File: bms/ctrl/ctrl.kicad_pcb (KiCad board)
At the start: 2 copper layers, 1 part

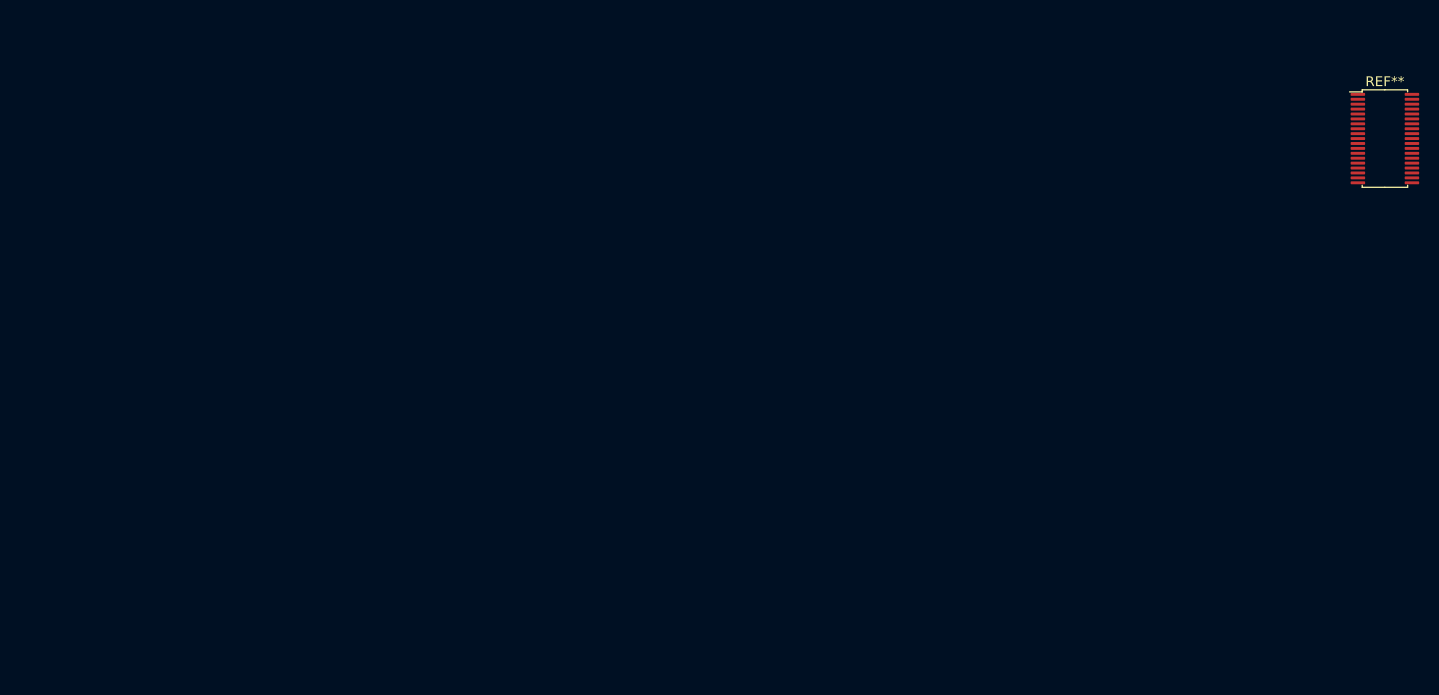
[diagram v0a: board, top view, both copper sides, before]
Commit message: BMS stuff update
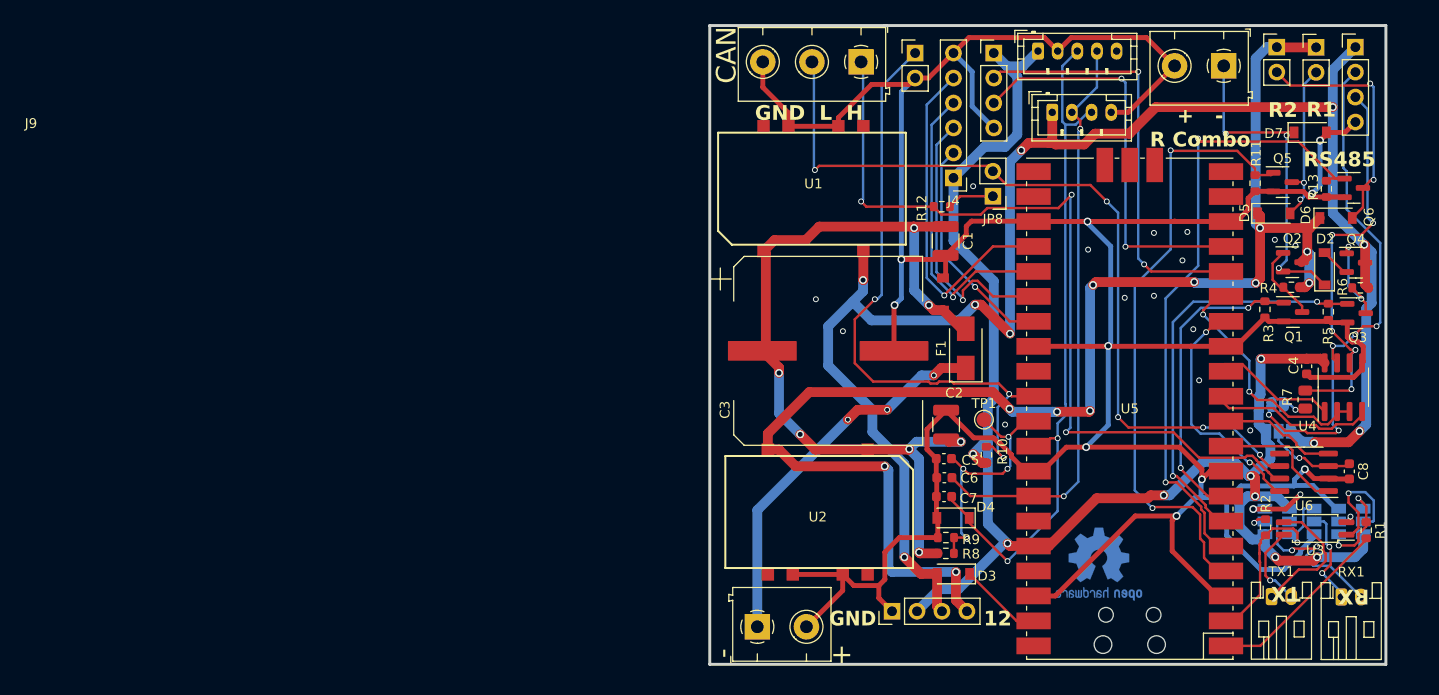
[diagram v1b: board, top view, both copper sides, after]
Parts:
- removed the REF** at (111.9, 82.9)
- added C1: CP_1µ_100V_0805, Resistor_SMD:R_1210_3225Metric, F.Cu at (67.2, 93.3)
- added C2: CP_1µ_100V_0805, Resistor_SMD:R_1210_3225Metric, F.Cu at (67.2, 112.0)
- added C3: CP_330µ_100V_1210, localstuff:CP_Elec_19x19, F.Cu at (55.2, 104.5)
- added C4: 100nF, Capacitor_SMD:C_0603_1608Metric, F.Cu at (103.9, 106.1)
- added C5: CP_100n_50V_0603, Capacitor_SMD:C_0603_1608Metric, F.Cu at (67.0, 115.5)
- added C6: CP_100n_50V_0603, Capacitor_SMD:C_0603_1608Metric, F.Cu at (67.1, 117.4)
- added C7: CP_100n_50V_0603, Capacitor_SMD:C_0603_1608Metric, F.Cu at (67.0, 119.3)
- added C8: CP_10µ_16V_0603, Capacitor_SMD:C_0603_1608Metric, F.Cu at (108.3, 116.8)
- added D1: D_TVS_70V, localstuff:SOD-123FL, F.Cu at (66.9, 98.7)
- added D2: 1N4148, Diode_SMD:D_SOD-123, F.Cu at (105.8, 96.2)
- added D3: D_Schottky, Diode_SMD:D_SOD-123, F.Cu at (68.0, 127.2)
- added D4: D_Zener_3V3, Diode_SMD:D_SOD-123, F.Cu at (68.0, 121.5)
- added D5: 1N4148, Diode_SMD:D_SOD-123, F.Cu at (100.6, 90.5)
- added D6: 1N4148, Diode_SMD:D_SOD-123, F.Cu at (106.9, 91.0)
- added D7: 1N4148, Diode_SMD:D_SOD-123, F.Cu at (104.3, 82.3)
- added F1: Polyfuse 100V, Diode_SMD:D_SMA, F.Cu at (69.2, 104.2)
- added J1: Conn_01x02_Female, localstuff:Conn_P5.0mm_2_Lumberg, F.Cu at (48.0, 132.6)
- added J10: Conn_LEM_3, Connector_JST:JST_PH_B5B-PH-K_1x05_P2.00mm_Vertical, F.Cu at (76.6, 74.0)
- added J11: Conn_01x02_Female, Connector_PinHeader_2.54mm:PinHeader_1x02_P2.54mm_Vertical, F.Cu at (100.9, 73.6)
- added J12: Conn_01x04, Connector_PinHeader_2.54mm:PinHeader_1x04_P2.54mm_Vertical, F.Cu at (61.8, 131.0)
- added J2: Conn_01x02_Female, localstuff:Conn_P5.0mm_2_Lumberg, F.Cu at (95.5, 75.5)
- added J3: ScrewTerminal, Connector_PinHeader_2.54mm:PinHeader_1x04_P2.54mm_Vertical, F.Cu at (108.9, 73.6)
- added J4: Conn_01x06, Connector_PinHeader_2.54mm:PinHeader_1x06_P2.54mm_Vertical, F.Cu at (68.0, 86.9)
- added J5: Conn_01x04, Connector_PinHeader_2.54mm:PinHeader_1x04_P2.54mm_Vertical, F.Cu at (72.1, 74.2)
- added J6: Conn_LEM_5, Connector_JST:JST_PH_B4B-PH-K_1x04_P2.00mm_Vertical, F.Cu at (78.0, 80.2)
- added J7: Conn_01x02_Male, Connector_PinHeader_2.54mm:PinHeader_1x02_P2.54mm_Vertical, F.Cu at (64.1, 74.2)
- added J8: Conn_01x02_Female, Connector_PinHeader_2.54mm:PinHeader_1x02_P2.54mm_Vertical, F.Cu at (104.9, 73.6)
- added J9: Conn_01x03, localstuff:Conn_P5.0mm_3_Lumberg, F.Cu at (58.6, 75.1)
- added JP1: SolderJumper_3_Bridged12, Jumper:SolderJumper-3_P1.3mm_Open_Pad1.0x1.5mm, B.Cu at (109.7, 121.9)
- added JP2: SolderJumper_3_Bridged12, Jumper:SolderJumper-3_P1.3mm_Open_Pad1.0x1.5mm, B.Cu at (107.2, 121.9)
- added JP3: SolderJumper_3_Bridged12, Jumper:SolderJumper-3_P1.3mm_Open_Pad1.0x1.5mm, B.Cu at (102.2, 121.9)
- added JP4: SolderJumper_3_Bridged12, Jumper:SolderJumper-3_P1.3mm_Open_Pad1.0x1.5mm, B.Cu at (104.7, 121.9)
- added JP5: SolderJumper_3_Bridged12, Jumper:SolderJumper-3_P1.3mm_Open_Pad1.0x1.5mm, B.Cu at (99.7, 121.9)
- added JP6: OptTermination, Jumper:SolderJumper-2_P1.3mm_Open_RoundedPad1.0x1.5mm, B.Cu at (101.0, 110.0)
- added JP7: CANBUS Volt Select, Jumper:SolderJumper-3_P1.3mm_Bridged12_RoundedPad1.0x1.5mm, B.Cu at (101.1, 112.7)
- added JP8: Jumper_2_Open, Connector_PinHeader_2.54mm:PinHeader_1x02_P2.54mm_Vertical, F.Cu at (72.0, 88.8)
- added Q1: DMN2058U-7, Package_TO_SOT_SMD:SOT-23, F.Cu at (102.5, 100.5)
- added Q2: XP221P0501TR-G, Package_TO_SOT_SMD:SOT-23, F.Cu at (102.5, 95.5)
- added Q3: DMN2058U-7, Package_TO_SOT_SMD:SOT-23, F.Cu at (109.0, 100.7)
- added Q4: XP221P0501TR-G, Package_TO_SOT_SMD:SOT-23, F.Cu at (109.0, 95.5)
- added Q5: DMN2058U-7, Package_TO_SOT_SMD:SOT-23, F.Cu at (101.5, 87.3)
- added Q6: DMN2058U-7, Package_TO_SOT_SMD:SOT-23, F.Cu at (108.7, 87.9)
- added R1: R_220_0603, Resistor_SMD:R_0603_1608Metric, F.Cu at (110.0, 122.8)
- added R10: R_10k_0603, Resistor_SMD:R_0603_1608Metric, F.Cu at (71.3, 115.1)
- added R11: R_1M_0603, Resistor_SMD:R_0603_1608Metric, F.Cu at (98.7, 87.4)
- added R12: R_120_0603, Resistor_SMD:R_0603_1608Metric, F.Cu at (66.8, 89.8)
- added R13: R_1M_0603, Resistor_SMD:R_0603_1608Metric, F.Cu at (106.0, 88.0)
- added R2: R_2k2_0603, Resistor_SMD:R_0603_1608Metric, F.Cu at (99.8, 122.5)
- added R3: R_1M_0603, Resistor_SMD:R_0603_1608Metric, F.Cu at (99.7, 100.3)
- added R4: R_1M_0603, Resistor_SMD:R_0603_1608Metric, F.Cu at (102.4, 98.0)
- added R5: R_1M_0603, Resistor_SMD:R_0603_1608Metric, F.Cu at (106.1, 100.5)
- added R6: R_1M_0603, Resistor_SMD:R_0603_1608Metric, F.Cu at (109.4, 98.1)
- added R7: 120R, Resistor_SMD:R_0805_2012Metric, F.Cu at (103.8, 109.5)
- added R8: R_750k_0603, Resistor_SMD:R_0603_1608Metric, F.Cu at (67.2, 125.1)
- added R9: R_36k_0603_1, Resistor_SMD:R_0603_1608Metric, F.Cu at (67.2, 123.5)
- added REF**: OSHW-Logo2_9.8x8mm_Copper, Symbol:OSHW-Logo2_9.8x8mm_Copper, B.Cu at (82.8, 126.2)
- added REF**: OSHW-Logo2_9.8x8mm_SilkScreen, Symbol:OSHW-Logo2_9.8x8mm_SilkScreen, B.Cu at (82.8, 126.2)
- added RX1: Conn_01x02_Male, Connector_JST:JST_PH_S2B-PH-K_1x02_P2.00mm_Horizontal, F.Cu at (107.5, 129.6)
- added TP1: TestPoint, TestPoint:TestPoint_Pad_D1.5mm, F.Cu at (71.1, 111.5)
- added TX1: Conn_01x02_Male, Connector_JST:JST_PH_S2B-PH-K_1x02_P2.00mm_Horizontal, F.Cu at (100.4, 129.5)
- added U1: STH05_5V, localstuff:STH05, F.Cu at (53.8, 88.0)
- added U2: STH05_12, localstuff:STH05, F.Cu at (54.2, 120.9)
- added U3: VOS618A, Package_SO:SOP-4_4.4x2.6mm_P1.27mm, F.Cu at (104.8, 122.6)
- added U4: SN65HVD75DR, Package_SO:SOIC-8_3.9x4.9mm_P1.27mm, F.Cu at (107.7, 108.2)
- added U5: Pico, pico:RPi_Pico_SMD_TH, F.Cu at (85.9, 110.4)
- added U6: SN65HVD1050D, Package_SO:SOIC-8_3.9x4.9mm_P1.27mm, F.Cu at (103.7, 116.9)
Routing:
- net GND: track 0.00 -> 386.3 mm, vias 0 -> 27
- net +5V: track 0.00 -> 173.5 mm, vias 0 -> 9
- net +3V3: track 0.00 -> 153.3 mm, vias 0 -> 8
- net +12V: track 0.00 -> 147.4 mm, vias 0 -> 11
- net Net-(J9-Pin_1): track 0.00 -> 85.5 mm, vias 0 -> 3
- net VBAT: track 0.00 -> 85.2 mm, vias 0 -> 7
- net Net-(J9-Pin_2): track 0.00 -> 83.6 mm, vias 0 -> 5
- net ADC_BAT_I: track 0.00 -> 69.1 mm, vias 0 -> 2
- net RESET: track 0.00 -> 64.4 mm, vias 0 -> 3
- net RELAY2: track 0.00 -> 63.3 mm, vias 0 -> 2
- net RELAY1: track 0.00 -> 62.3 mm, vias 0 -> 2
- net ADC_REF_I: track 0.00 -> 59.6 mm, vias 0 -> 2
- net Net-(J3-Pin_2): track 0.00 -> 53.2 mm, vias 0 -> 5
- net I2C0_SDA: track 0.00 -> 42.5 mm, vias 0 -> 2
- net Net-(J3-Pin_3): track 0.00 -> 41.7 mm, vias 0 -> 5
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- added copper zone on B.Cu, net GND
- added copper zone on F.Cu, net GND
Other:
- board outline added: 68.8 x 65 mm
- board text added: "+"
- board text added: "+ - R Combo"
- board text added: "-"
- board text added: "12"
- board text added: "5v CAN 3.3v"
- board text added: "CAN"
- board text added: "GND"
- board text added: "GND L H"
- board text added: "MoaT comm"
- board text added: "MoaT/diyBMS battery controller V 1.0"
- board text added: "R1"
- board text added: "R2"
- board text added: "RS485"
- board text added: "RS485 term"
- board text added: "RX"
- board text added: "TX"
- board text added: "diyBMS comm"
